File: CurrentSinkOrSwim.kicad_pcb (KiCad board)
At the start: 2 copper layers, 43.2 x 53.3 mm, 23 parts, among them P101 CONN_01X03, P102 CONN_01X02, P103 CONN_01X02, P201 CONN_01X01, Q201 BUK9575, U201 LMV358, U401 LM2931D-R

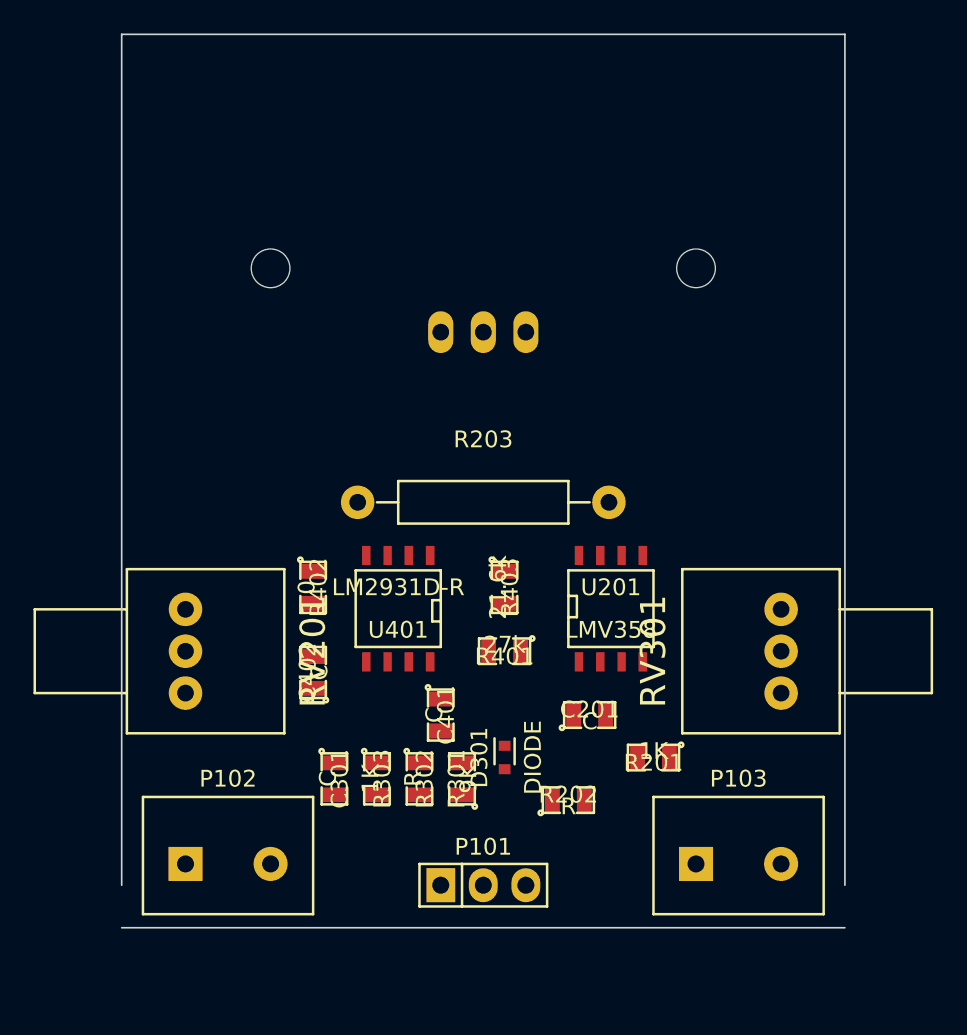
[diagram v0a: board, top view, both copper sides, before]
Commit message: Initial layout
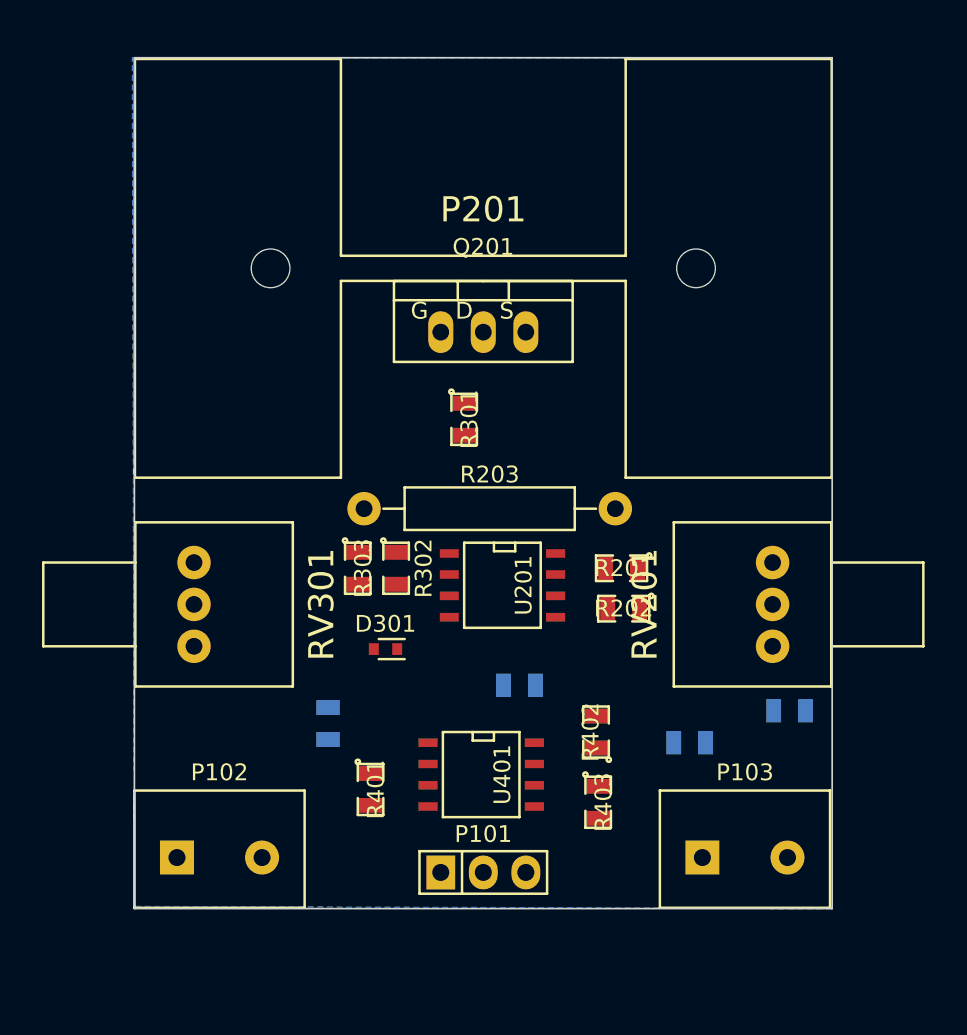
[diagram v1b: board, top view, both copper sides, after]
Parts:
- C201, C301, C401, C402: moved to B.Cu
- P201, Q201: moved to F.Cu
- moved RV301 35.2 mm to (99.6, 74.7), turned to 270 degrees
- moved RV201 35.2 mm to (134.1, 74.7), turned to 90 degrees
- moved R301 21.5 mm to (115.7, 63.6), turned to 270 degrees
- moved C301 21.3 mm to (129.2, 82.9), turned to 0 degrees
- moved R402 19.0 mm to (123.6, 82.3), turned to 90 degrees
- moved R403 14.0 mm to (123.7, 86.5)
- moved R302 12.7 mm to (111.6, 72.5)
- moved R303 12.6 mm to (109.3, 72.5)
- moved C402 12.3 mm to (119.0, 79.5), turned to 180 degrees
- moved C201 11.9 mm to (135.1, 81.0)
- moved R202 11.9 mm to (125.2, 74.9), turned to 180 degrees
- moved R401 11.5 mm to (110.1, 85.7), turned to 270 degrees
- moved R201 11.5 mm to (125.1, 72.5)
- moved U401 11.1 mm to (116.7, 84.8), turned to 270 degrees
- moved D301 9.62 mm to (111.0, 77.3), turned to 0 degrees
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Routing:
- added copper zone on B.Cu, net (none)
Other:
- board size 43.2 x 53.3 mm -> 41.7 x 50.8 mm

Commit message: First cut of layout in preperation for the final session
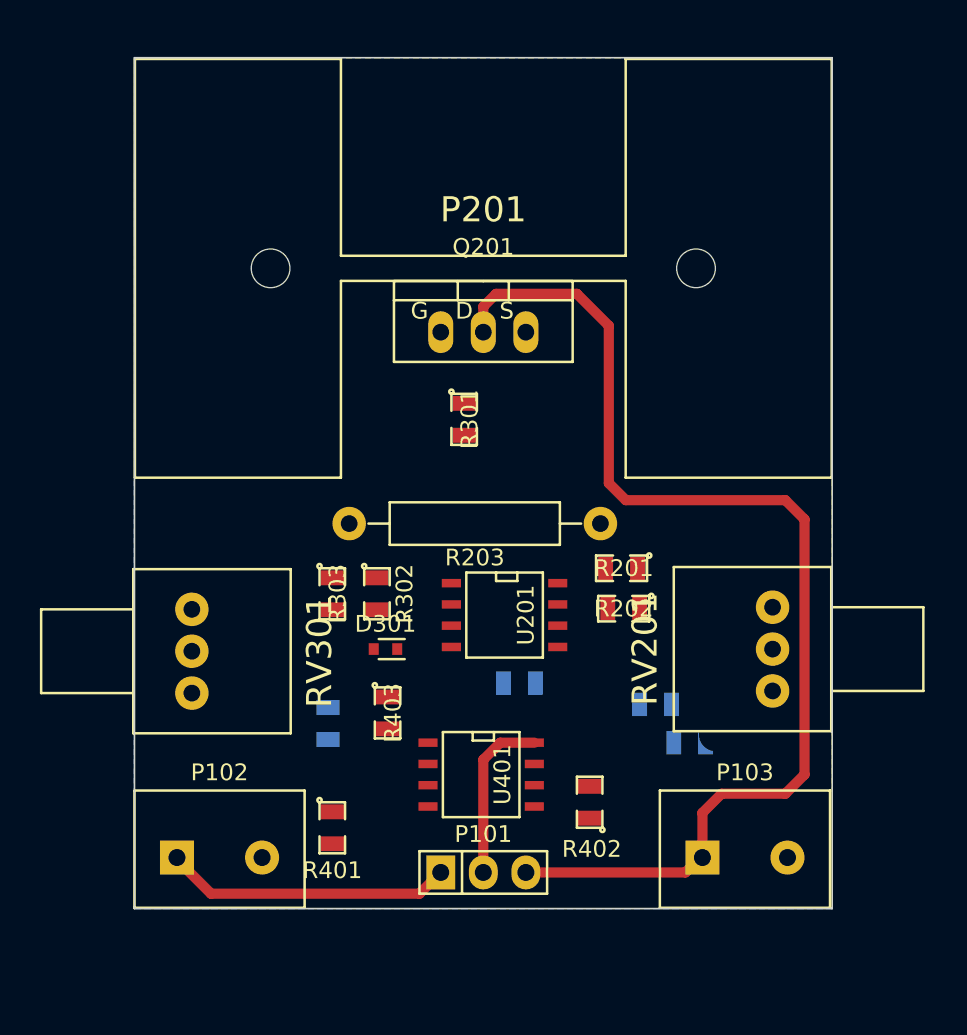
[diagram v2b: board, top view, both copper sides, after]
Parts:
- R202: value R -> 68K
- R302: value R -> 28.7K
- RV201, RV301: value POT -> 10K
- moved R403 13.7 mm to (111.1, 81.2)
- moved C201 8.01 mm to (127.1, 80.6)
- moved R402 4.21 mm to (123.2, 86.5)
- moved R401 3.23 mm to (107.8, 88.0)
- moved RV301 2.80 mm to (99.4, 77.5)
- moved RV201 2.67 mm to (134.1, 77.3)
- moved R303 2.16 mm to (107.8, 74.0)
- moved R302 1.91 mm to (110.5, 74.0)
- moved U201 1.78 mm to (118.1, 75.3)
- moved R203 1.26 mm to (116.3, 69.8), turned to 180 degrees
- moved C402 0.13 mm to (119.0, 79.4), turned to 0 degrees
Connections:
- R202 pad 1: Net-(R202-Pad1) -> 2.7V
- R202 pad 2: GND -> Net-(R202-Pad2)
- R301 pad 2: Net-(R301-Pad2) -> /Voltage Control/0-2v
- R302 pad 1: Net-(R302-Pad1) -> 2.7V
- R302 pad 2: GND -> /Voltage Control/0-2v
- R303 pad 1: Net-(R301-Pad2) -> /Voltage Control/0-2v
- R401 pad 1: Net-(R401-Pad1) -> 2.7V
- RV201 pad 1: Net-(RV201-Pad1) -> Net-(R202-Pad2)
- RV201 pad 2: 2.7V -> GND
- RV201 pad 3: Net-(R202-Pad1) -> Net-(RV201-Pad3)
- RV301 pad 2: 2.7V -> /Voltage Control/0-2v
- RV301 pad 3: Net-(R302-Pad1) -> GND
- U201 pad 3: Net-(R202-Pad1) -> Net-(R202-Pad2)
- U201 pad 5: Net-(R302-Pad1) -> /Voltage Control/0-2v
- U201 pad 6: Net-(R301-Pad2) -> /Voltage Control/0-2v
- U401 pad 1: Net-(U401-Pad1) -> 2.7V
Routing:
- net /Current Control/Current_Sink+: track 0.00 -> 68.0 mm
- net Net-(P101-Pad1): track 0.00 -> 17.2 mm
- net /Power Regulation/Vin: track 0.00 -> 10.2 mm
- added copper zone on B.Cu, net GND
- removed copper zone on B.Cu, net (none)
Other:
- net class Power added: clearance 0.3048, trace_width 0.6096, via_dia 1.143, via_drill 0.762

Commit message: Routing and fixing schematic checkpoint
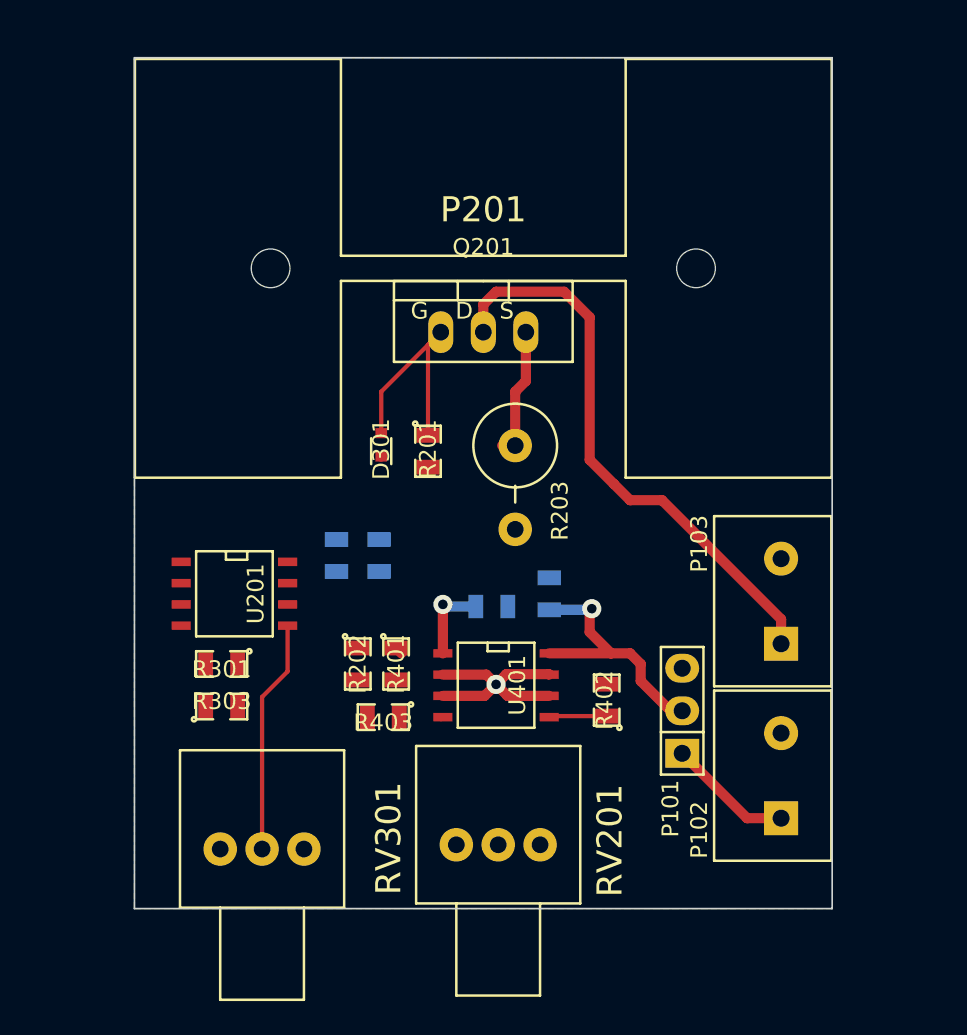
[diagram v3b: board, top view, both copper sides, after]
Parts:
- removed C301: C, SMD_Packages:SMD-0805
- R203: footprint Resistors_ThroughHole:Resistor_Horizontal_RM15mm -> Resistors_ThroughHole:Resistor_Vertical_RM5mm
- R302: moved to B.Cu
- moved P102 33.9 mm to (134.6, 84.9), turned to 90 degrees
- moved C201 21.0 mm to (108.1, 71.8), turned to 270 degrees
- moved R301 20.6 mm to (101.2, 78.2), turned to 180 degrees
- moved RV201 20.1 mm to (117.7, 89.0), turned to 0 degrees
- moved R202 16.2 mm to (109.3, 78.2), turned to 270 degrees
- moved U201 16.2 mm to (102.0, 74.0)
- moved P103 15.5 mm to (134.6, 74.5), turned to 90 degrees
- moved C401 15.3 mm to (120.8, 74.0)
- moved P101 15.3 mm to (128.7, 81.0), turned to 90 degrees
- moved R201 13.5 mm to (113.5, 65.5), turned to 270 degrees
- moved RV301 12.5 mm to (103.6, 89.3), turned to 0 degrees
- moved D301 12.2 mm to (110.7, 65.2), turned to 270 degrees
- moved R401 10.5 mm to (111.6, 78.2)
- moved R303 9.43 mm to (101.2, 80.8), turned to 0 degrees
- moved R402 6.18 mm to (124.2, 80.4)
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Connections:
- R301 pad 2: /Voltage Control/0-2v -> /Voltage Control/0-2v_FeedBack
- R303 pad 1: /Voltage Control/0-2v -> /Voltage Control/0-2v_FeedBack
- U201 pad 6: /Voltage Control/0-2v -> /Voltage Control/0-2v_FeedBack
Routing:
- net /Current Control/Current_Sink+: track 68.0 -> 34.3 mm
- net /Current Control/FET_GATE: track 0.00 -> 14.0 mm
- net /Voltage Control/0-2v: track 0.00 -> 14.0 mm
- net GND: track 0.00 -> 13.8 mm, vias 0 -> 1
- net Net-(P101-Pad1): track 17.2 -> 7.51 mm
- net Net-(Q201-PadS): track 0.00 -> 7.81 mm
- net 2.7V: track 0.00 -> 5.57 mm, vias 0 -> 1
- net /Power Regulation/Vin: track 10.2 -> 15.8 mm, vias 0 -> 1
- net Net-(R402-Pad1): track 0.00 -> 3.46 mm
